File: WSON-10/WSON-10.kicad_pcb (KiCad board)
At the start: 2 copper layers, 13.8 x 16.4 mm, 3 parts, among them J1 Conn_01x06_Male, J2 Conn_01x06_Male, U1 TPS62177DQC

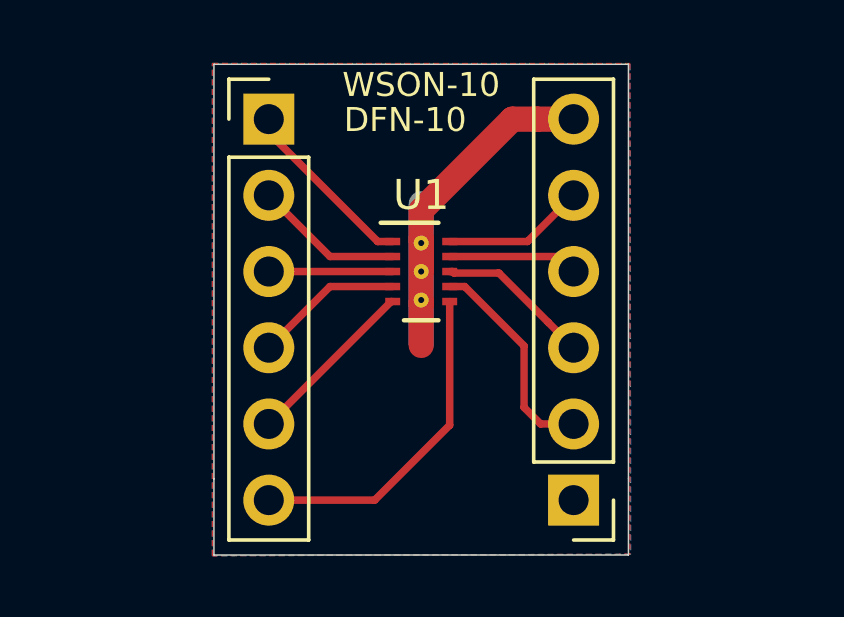
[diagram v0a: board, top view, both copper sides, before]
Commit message: get the WSON-10 Working
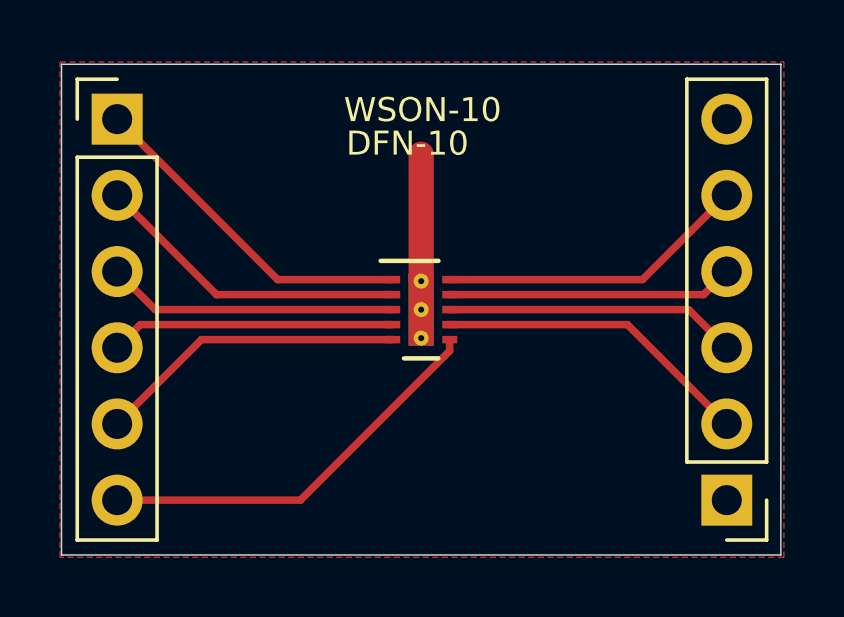
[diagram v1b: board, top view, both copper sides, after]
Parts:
- moved J2 5.11 mm to (77.3, 64.5)
- moved J1 5.05 mm to (57.0, 51.8)
- moved U1 1.27 mm to (67.2, 58.2)
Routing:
- net PAD: track 12.7 -> 4.23 mm
- net VOS: track 4.77 -> 10.4 mm
- net EN: track 4.13 -> 9.71 mm
- net VIN: track 4.97 -> 10.6 mm
- net PGND: track 6.08 -> 11.4 mm
- net SW: track 4.34 -> 9.55 mm
- net nSLEEP: track 5.18 -> 9.76 mm
- net FB: track 5.82 -> 10.3 mm
- net NC: track 4.97 -> 9.50 mm
- net PG: track 7.23 -> 10.6 mm
- net AGND: track 11.2 -> 13.5 mm
- removed copper zone on B.Cu, net PAD
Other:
- board size 13.8 x 16.4 mm -> 24 x 16.4 mm
